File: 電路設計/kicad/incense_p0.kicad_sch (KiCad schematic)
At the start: 13 parts, among them J1 K型熱電偶, J2 12V 3A 變壓器, K1 電磁鐵 ×4（理香，脈衝驅動）, M1 5015 渦輪風扇 12V 0.2A, M2 超音波霧化模組 12V（冷霧，無明火）, U2 SCD41 CO2 (0x62) - I2C1 埠, U3 GY-SHT31-D (0x44) - I2C2 埠, U5 MAX6675 熱電偶介面, U6 D4184 MOSFET 模組, U7 I2C 8路 MOSFET 驅動板

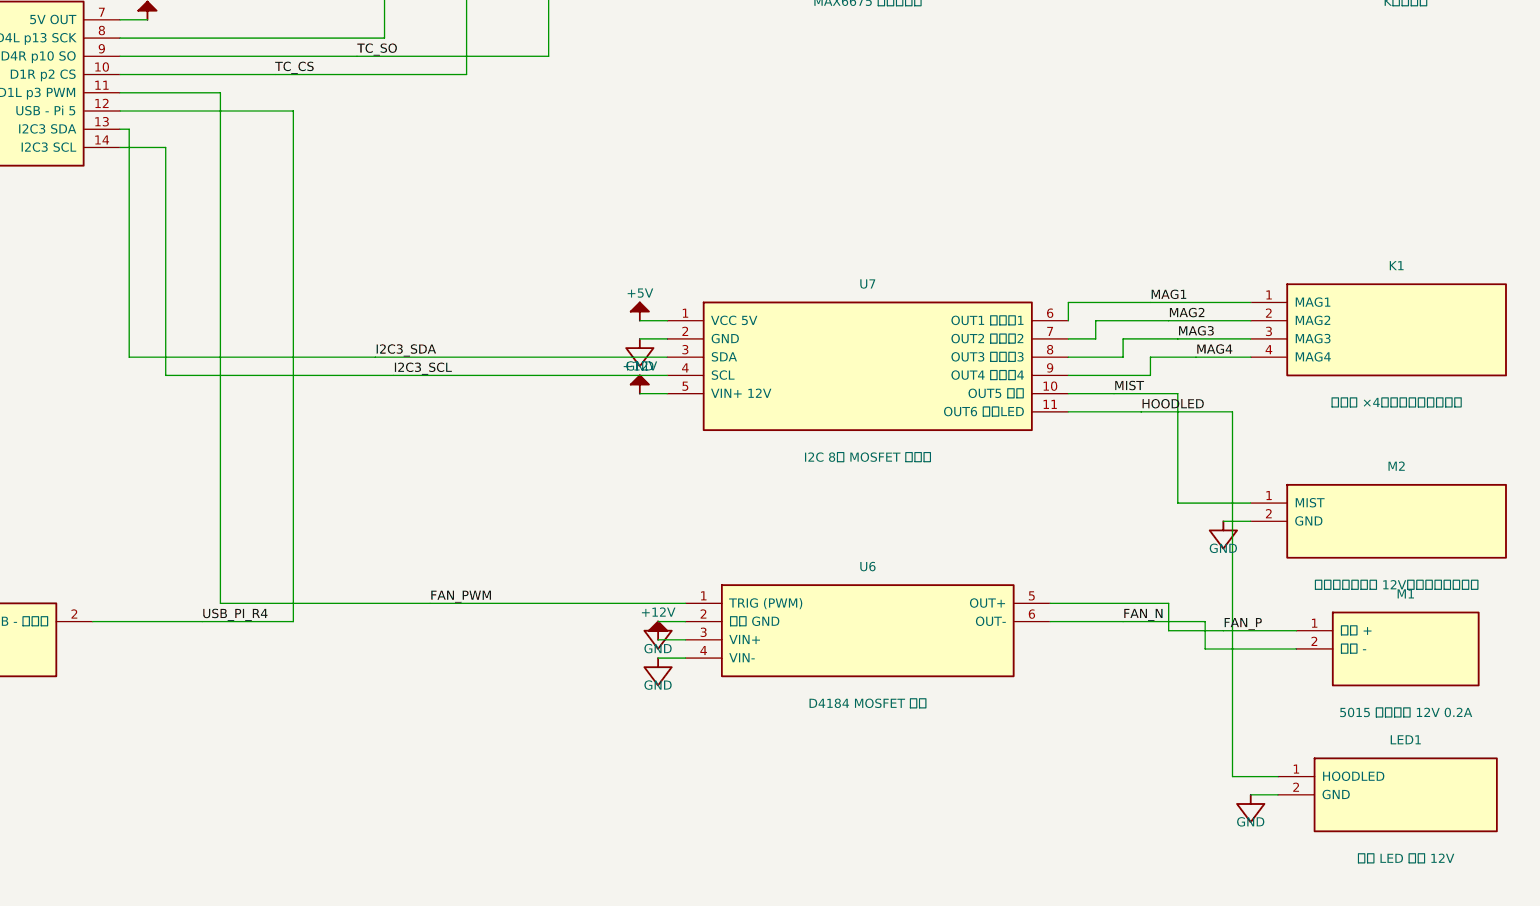
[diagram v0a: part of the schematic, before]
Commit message: auto-sync 2026-08-16 12:39
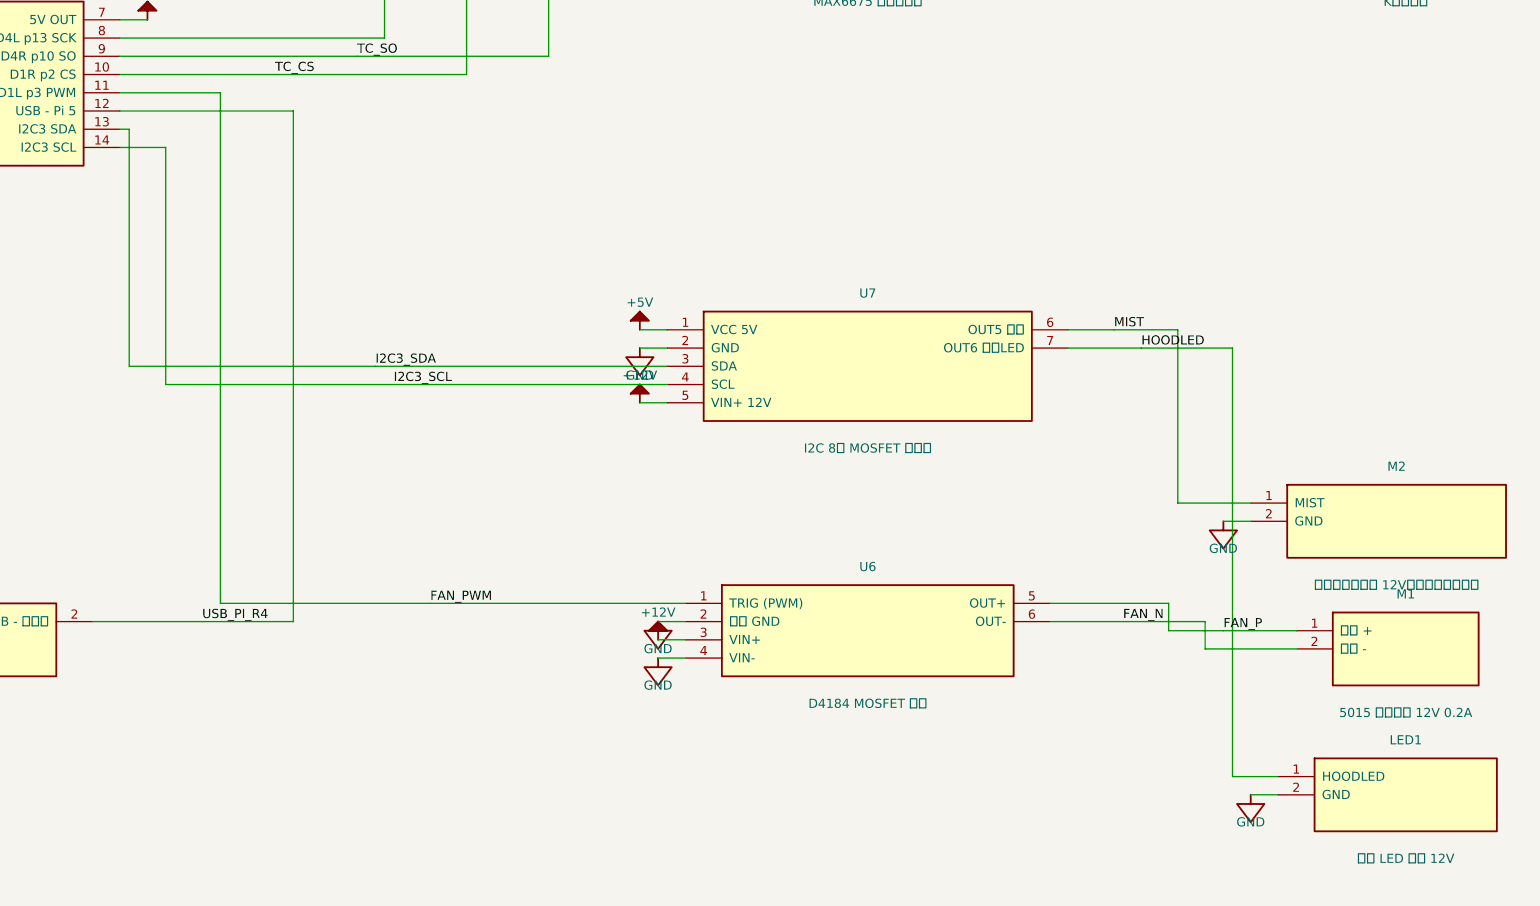
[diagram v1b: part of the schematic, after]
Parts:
- removed K1: 電磁鐵 ×4（理香，脈衝驅動）, symbol incense:Solenoid-Array
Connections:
- net MAG1 is gone; now on net MIST: U7.6 (OUT5 霧化)
- net MAG2 is gone; now on net HOODLED: U7.7 (OUT6 罩內LED)
- net HOODLED: no longer U7.11 (OUT6 罩內LED)
- net MIST: no longer U7.10 (OUT5 霧化)
- removed net MAG3: U7.8 (OUT3 電磁鐵3)
- removed net MAG4: U7.9 (OUT4 電磁鐵4)
